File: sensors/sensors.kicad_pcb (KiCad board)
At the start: 2 copper layers, 42.4 x 20.7 mm, 22 parts, among them J1 Conn_01x16_Male, J2 Conn_01x16_Male, SW1 SW_DIP_x02, U1 IST8310, U2 MPU-9250, U3 MS5611-01BA, U4 ICM-20602

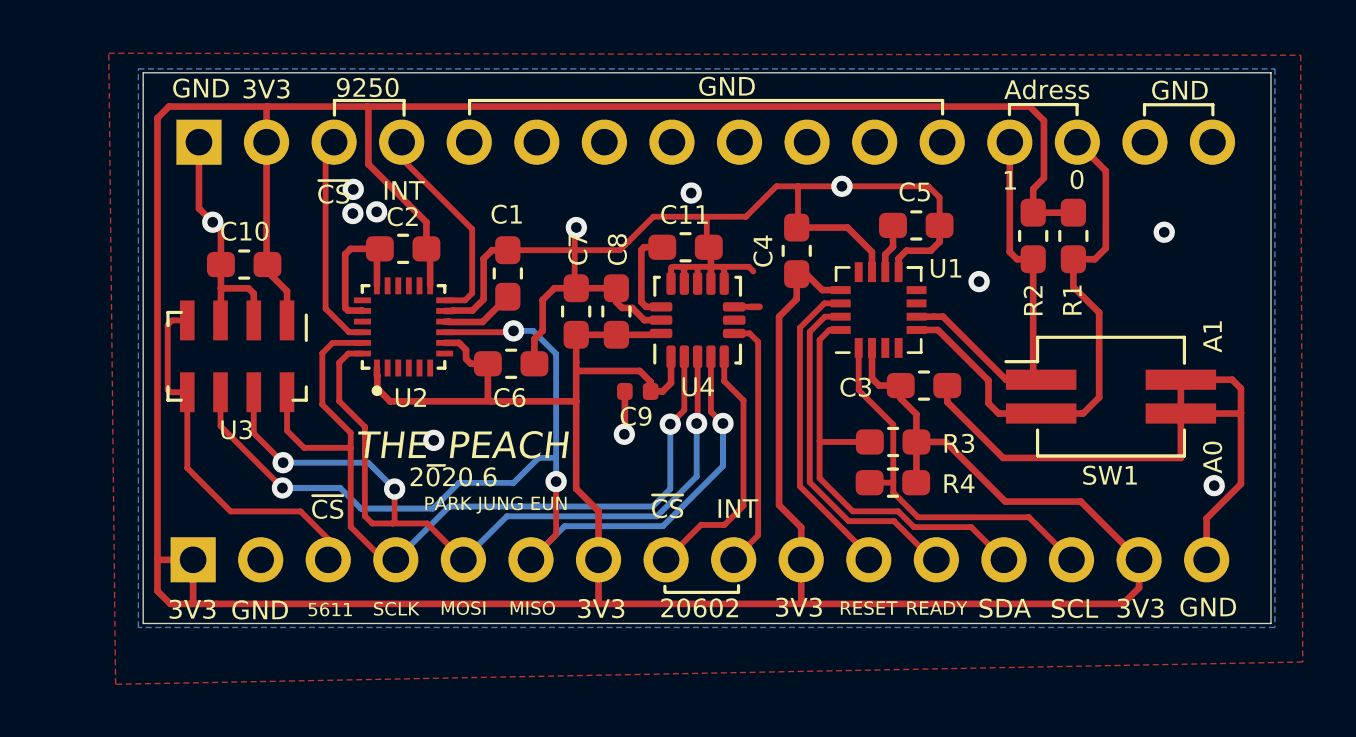
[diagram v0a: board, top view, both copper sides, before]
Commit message: 6월9일
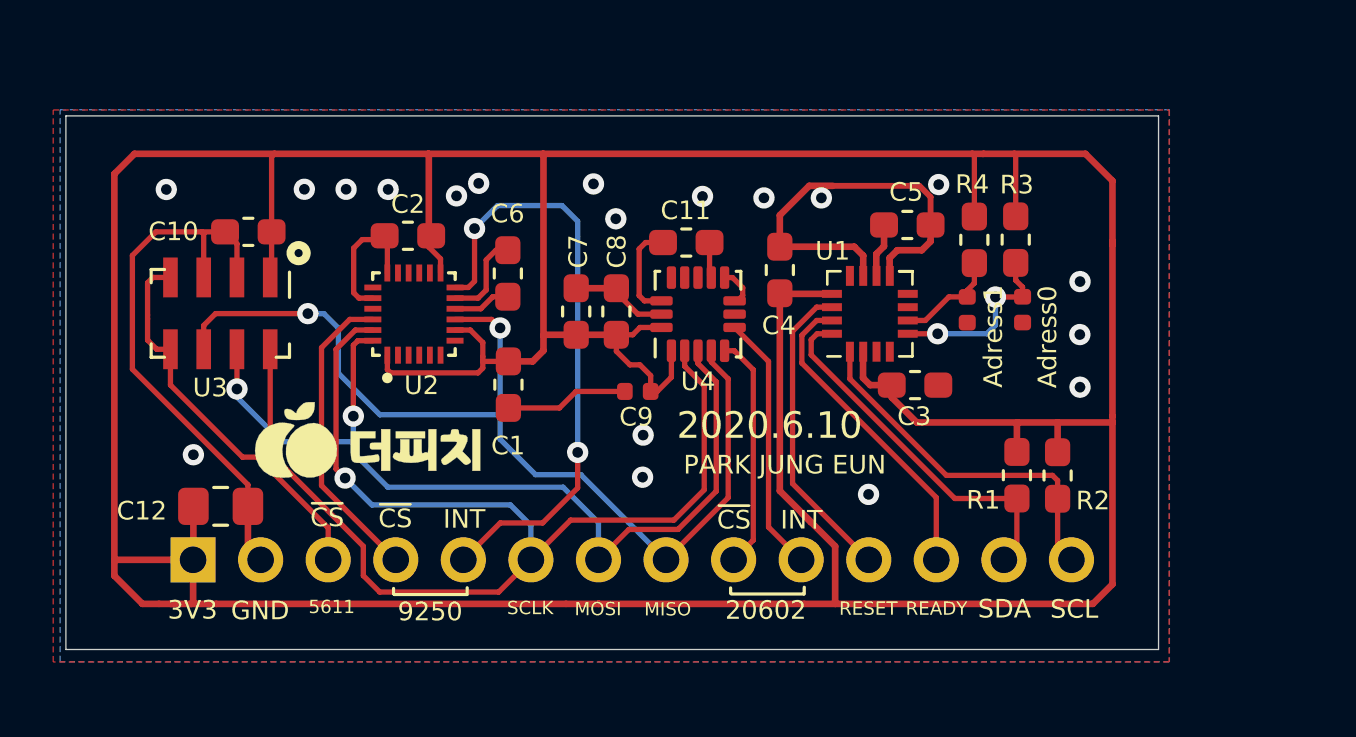
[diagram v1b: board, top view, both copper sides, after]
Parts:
- removed J2: Conn_01x16_Male, Connector_PinHeader_2.54mm:PinHeader_1x16_P2.54mm_Vertical
- removed SW1: SW_DIP_x02, Button_Switch_SMD:SW_DIP_SPSTx02_Slide_KingTek_DSHP02TJ_W5.25mm_P1.27mm_JPin
- added Adress0: Jumper, Capacitor_SMD:C_0402_1005Metric, F.Cu at (183.3, 62.7)
- added Adress1: Jumper, Capacitor_SMD:C_0402_1005Metric, F.Cu at (181.2, 62.7)
- added C12: C, Capacitor_SMD:C_0805_2012Metric_Pad1.15x1.40mm_HandSolder, F.Cu at (153.1, 70.1)
- added G***: LOGO, sensors:THEpeach, F.Cu at (158.7, 67.5)
- J1: value Conn_01x16_Male -> Conn_01x14_Male; footprint Connector_PinHeader_2.54mm:PinHeader_1x16_P2.54mm_Vertical -> Connector_PinHeader_2.54mm:PinHeader_1x14_P2.54mm_Vertical
- moved R2 6.20 mm to (184.6, 68.9), turned to 90 degrees
- moved R1 4.82 mm to (183.1, 68.9), turned to 90 degrees
- moved R4 2.22 mm to (181.5, 60.1)
- moved R3 2.17 mm to (183.0, 60.0)
- moved U3 1.73 mm to (153.1, 62.8)
- moved C10 1.24 mm to (154.2, 59.8)
- moved C4 0.96 mm to (174.1, 61.2)
- moved C1 0.79 mm to (163.9, 65.5), turned to 270 degrees
- moved U2 0.62 mm to (160.4, 62.8)
- moved C2 0.52 mm to (160.2, 59.9)
- moved U1 0.36 mm to (177.5, 62.8)
- moved C3 0.34 mm to (179.2, 65.5)
- moved C5 0.34 mm to (178.9, 59.5)
- moved U4 0.23 mm to (171.1, 62.8)
- moved C11 0.18 mm to (170.6, 60.2)
- renumbered R3 to R1, R4 to R2, R1 to R3, R2 to R4
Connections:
- net ADRESS0 renamed Net-(JP1-Pad1)
- net ADRESS1 renamed Net-(JP2-Pad1)
- J1 pad 10: VDD -> INT_20602
- J1 pad 4: SCLK -> ~CS_9250
- J1 pad 5: MOSI -> INT_9250
- J1 pad 6: MISO -> SCLK
- J1 pad 7: VDD -> MOSI
- J1 pad 8: ~CS_20602 -> MISO
- J1 pad 9: INT_20602 -> ~CS_20602
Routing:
- net GND: track 93.1 -> 56.8 mm, vias 12 -> 19
- net INT_9250: track 7.92 -> 22.7 mm, vias 0 -> 2
- net SCLK: track 31.6 -> 45.9 mm
- net Net-(JP1-Pad1): track 20.6 -> 6.89 mm, vias 0 -> 2
- net Net-(JP2-Pad1): track 15.4 -> 3.98 mm
- net VDD: track 176.9 -> 182.8 mm
- net ~CS_9250: track 8.14 -> 12.0 mm
- net MISO: track 41.7 -> 38.8 mm, vias 4 -> 2
- net SDA: track 16.3 -> 13.9 mm
- net ~CS_5611: track 14.1 -> 16.0 mm
- net ~CS_20602: track 10.4 -> 8.83 mm
- net READY: track 13.0 -> 11.9 mm
- net SCL: track 14.6 -> 13.6 mm
- net MOSI: track 35.3 -> 34.5 mm, vias 3 -> 2
- net Net-(C6-Pad1): track 2.77 -> 2.17 mm
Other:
- board size 42.4 x 20.7 mm -> 41.1 x 20.1 mm
- board text added: "2020.6.10"
- board text removed: "0"
- board text removed: "1"
- board text removed: "2020.6"
- board text removed: "A0"
- board text removed: "A1"
- board text removed: "Adress"
- board text removed: "THE_PEACH"
